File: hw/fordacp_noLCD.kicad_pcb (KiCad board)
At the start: 2 copper layers, 39.7 x 28.7 mm, 33 parts, among them IC1 ATMEGA2560-A, P1 CONN_02X06, U1 SP3485CN, U2 AP1117D50, U3 BLK-MD-SPK-B, U4 XS3860, Y1 16MHz

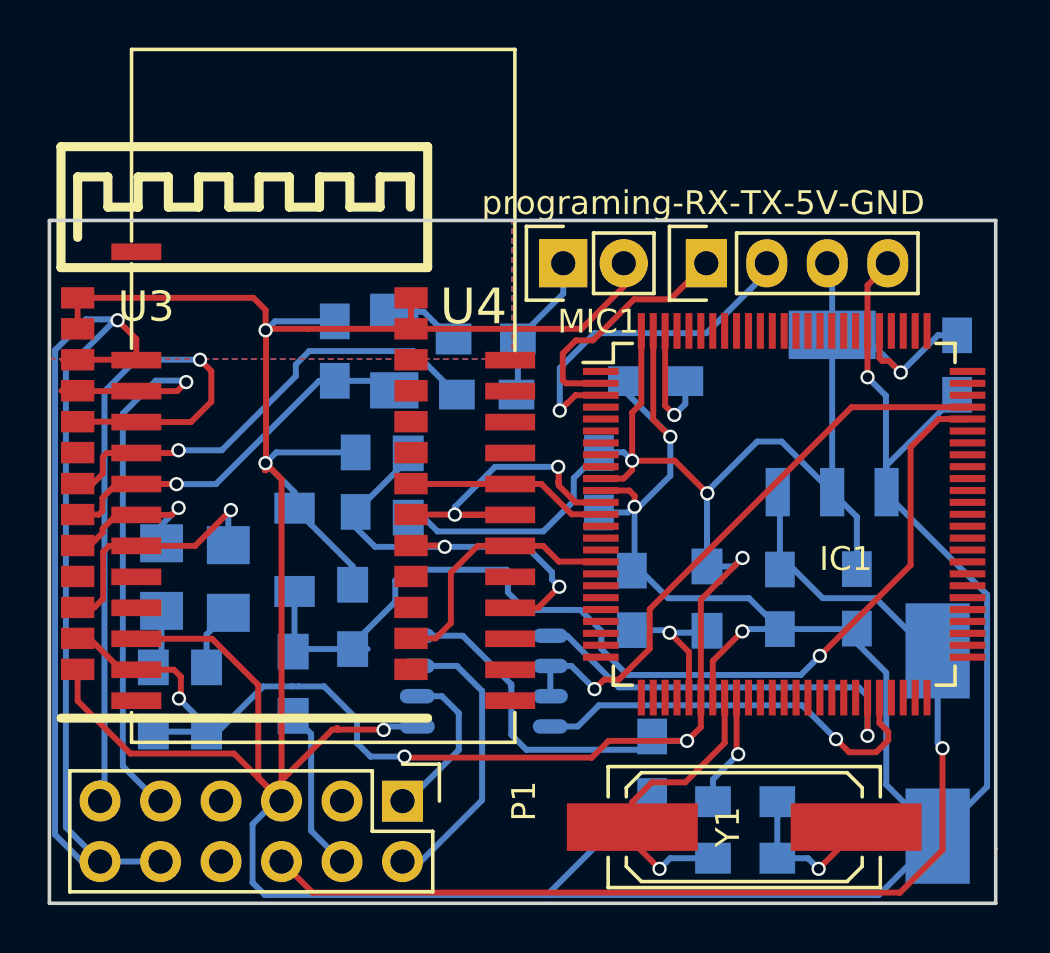
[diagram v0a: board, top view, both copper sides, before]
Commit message: update
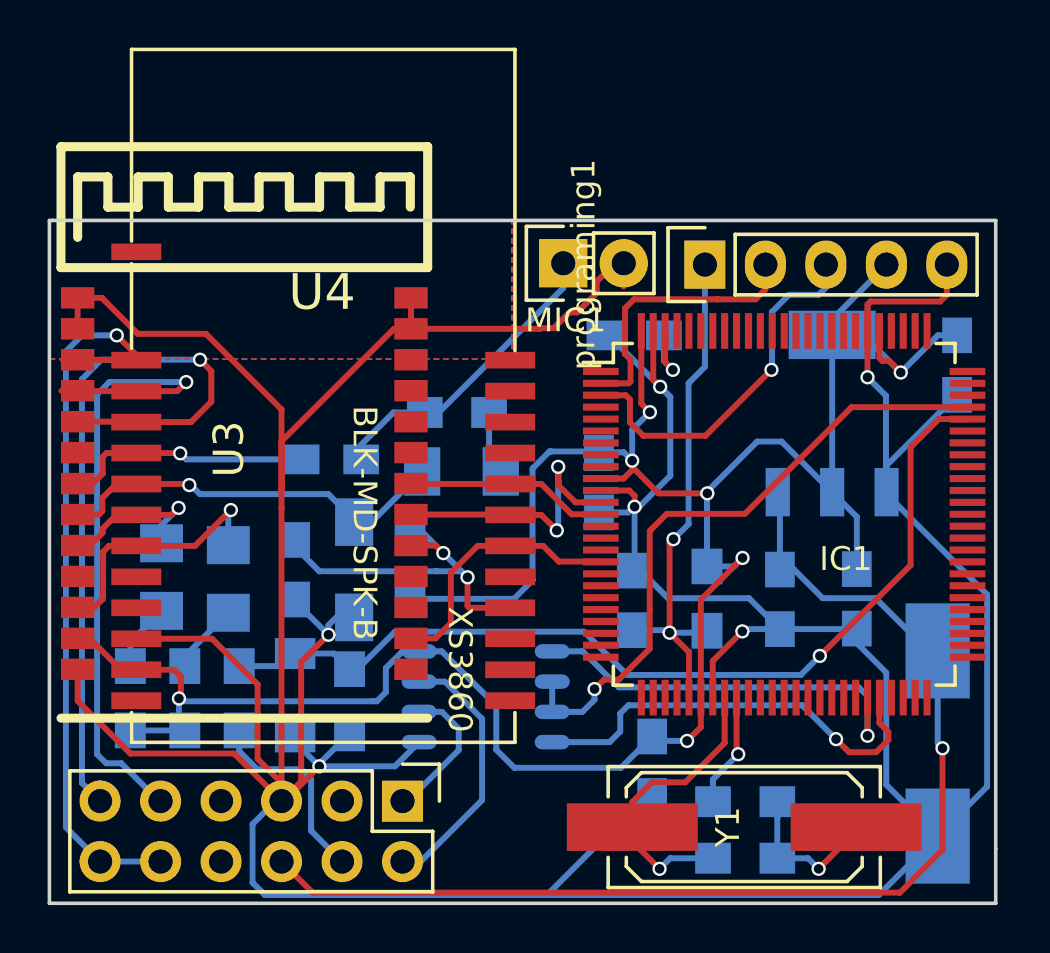
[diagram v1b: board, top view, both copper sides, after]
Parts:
- removed programing-RX-TX-5V-GND: CONN_01X02, Pin_Headers:Pin_Header_Straight_1x04
- added programing1: CONN_01X05, Pin_Headers:Pin_Header_Straight_1x05, F.Cu at (142.2, 90.2)
- C10, C11: value 2u2/10V -> 1u/16V
- C4: footprint Capacitors_SMD:C_0805_HandSoldering -> Capacitors_SMD:C_1206_HandSoldering
- R8, R9: value 4k7 -> 10k
- moved C4 9.22 mm to (127.5, 103.1), turned to 270 degrees
- moved C3 7.06 mm to (126.6, 98.4)
- moved D3 6.11 mm to (125.0, 108.3), turned to 270 degrees
- moved L1 5.79 mm to (132.0, 98.9), turned to 0 degrees
- moved C11 4.47 mm to (125.0, 103.1), turned to 270 degrees
- moved R7 3.55 mm to (127.3, 108.6), turned to 90 degrees
- moved R9 3.41 mm to (129.9, 102.9)
- moved R1 3.31 mm to (131.8, 96.5), turned to 0 degrees
- moved R6 2.35 mm to (122.7, 108.5)
- moved C9 2.12 mm to (139.3, 93.2)
- moved R4 0.97 mm to (118.1, 108.5)
- moved R5 0.92 mm to (120.4, 108.5)
- moved U1 0.66 mm to (133.0, 108.4)
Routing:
- net GNDA: track 58.4 -> 32.8 mm
- net /ARD_RESET: track 6.30 -> 22.4 mm, vias 1 -> 2
- net /MIC: track 19.8 -> 10.6 mm
- net +5V: track 120.0 -> 113.3 mm
- net Net-(C3-Pad1): track 6.33 -> 12.9 mm
- net GND: track 213.0 -> 219.4 mm, vias 7 -> 6
- net /ENABLE_5V: track 43.6 -> 40.4 mm
- net /BT_TX: track 14.8 -> 12.0 mm
- net /AUXINL: track 25.8 -> 28.2 mm
- net /RS485_ENA: track 25.1 -> 27.2 mm
- net /MIC_BIAS: track 16.1 -> 18.0 mm
- net /ARD_AREF: track 5.30 -> 3.41 mm
- net /AUXINR: track 30.5 -> 32.3 mm
- net /ENABLE: track 6.97 -> 8.38 mm
- net /RX0: track 10.4 -> 11.8 mm
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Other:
- board text added: "5V"
- board text added: "BLK-MD-SPK-B"
- board text added: "GND"
- board text added: "MIC"
- board text added: "RX"
- board text added: "TX"
- board text added: "XS3860"
